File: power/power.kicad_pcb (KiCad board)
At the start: 2 copper layers, 49.5 x 48.3 mm, 7 parts, among them J1 Conn_01x08_Male, J2 Conn_01x08_Male, J3 Jack-DC

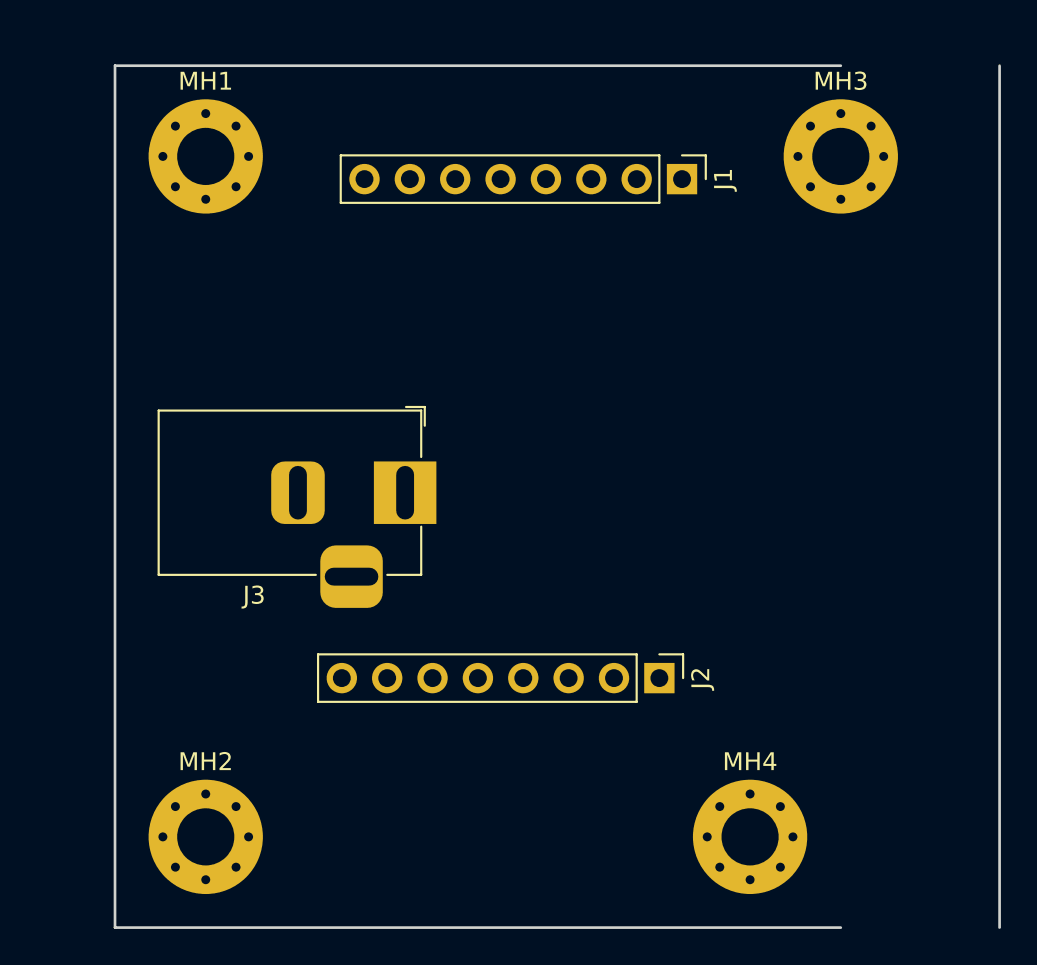
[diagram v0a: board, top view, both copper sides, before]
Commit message: Ready
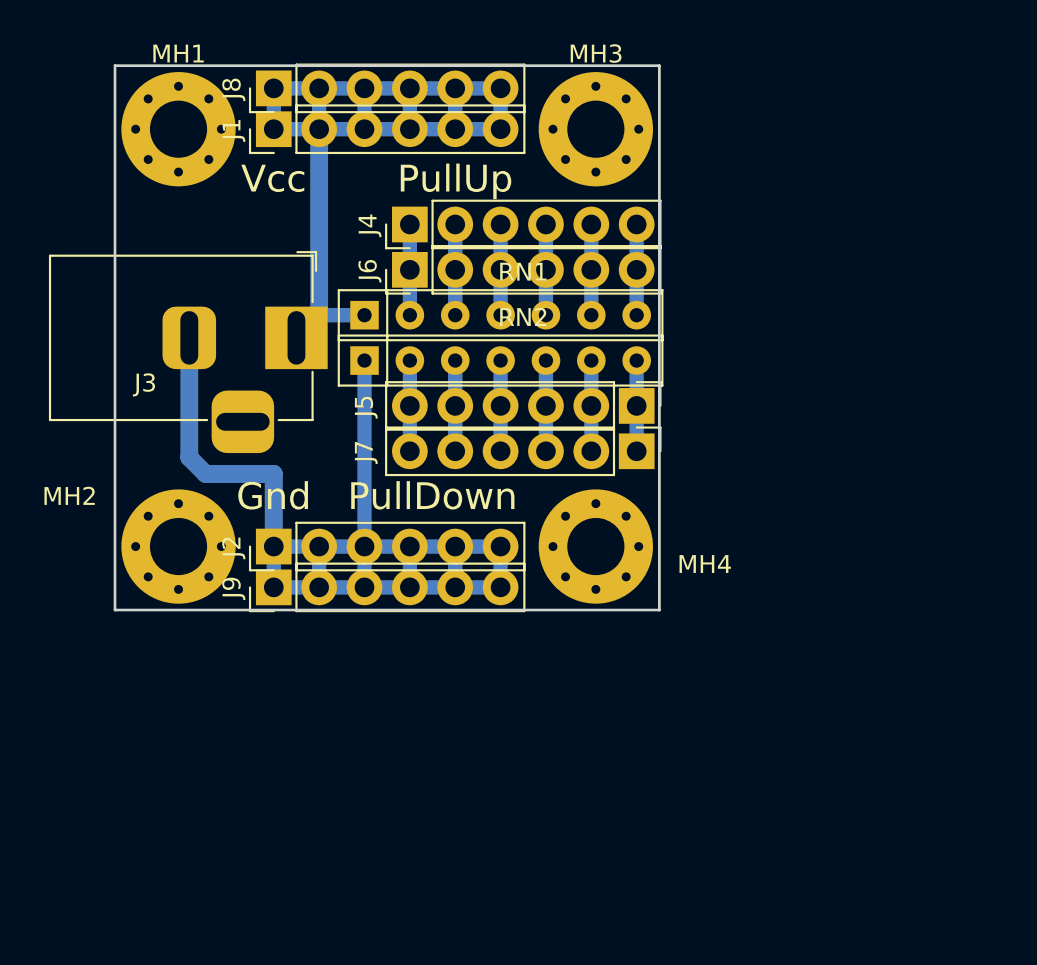
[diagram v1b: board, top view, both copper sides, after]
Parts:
- added J4: Conn_01x06_Male, MyLib:PinHeader_1x06_P2.54mm_Vertical_BigHoles, F.Cu at (148.6, 43.2)
- added J5: Conn_01x06_Male, MyLib:PinHeader_1x06_P2.54mm_Vertical_BigHoles, F.Cu at (161.3, 53.3)
- added J6: Conn_01x06_Male, MyLib:PinHeader_1x06_P2.54mm_Vertical_BigHoles, F.Cu at (148.6, 45.7)
- added J7: Conn_01x06_Male, MyLib:PinHeader_1x06_P2.54mm_Vertical_BigHoles, F.Cu at (161.3, 55.9)
- added J8: Conn_01x06_Male, MyLib:PinHeader_1x06_P2.54mm_Vertical_BigHoles, F.Cu at (141.0, 35.6)
- added J9: Conn_01x06_Male, MyLib:PinHeader_1x06_P2.54mm_Vertical_BigHoles, F.Cu at (141.0, 63.5)
- added RN1: R_Network06, Resistor_THT:R_Array_SIP7, F.Cu at (146.1, 48.3)
- added RN2: R_Network06, Resistor_THT:R_Array_SIP7, F.Cu at (146.1, 50.8)
- J1, J2: value Conn_01x08_Male -> Conn_01x06_Male; footprint Connector_PinHeader_2.54mm:PinHeader_1x08_P2.54mm_Vertical -> MyLib:PinHeader_1x06_P2.54mm_Vertical_BigHoles
- moved J1 23.0 mm to (141.0, 37.8), turned to 90 degrees
- moved J2 22.8 mm to (141.0, 61.2), turned to 90 degrees
- moved MH4 18.4 mm to (159.0, 61.2)
- moved MH2 16.3 mm to (135.6, 61.2)
- moved MH3 13.8 mm to (159.0, 37.8)
- moved J3 10.6 mm to (142.2, 49.5)
- moved MH1 2.16 mm to (135.6, 37.8)
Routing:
- net GND: track 0.00 -> 65.4 mm
- net VCC: track 0.00 -> 53.9 mm
- net Net-(J5-Pad6): track 0.00 -> 5.08 mm
- net Net-(J5-Pad5): track 0.00 -> 5.08 mm
- net Net-(J5-Pad4): track 0.00 -> 5.08 mm
- net Net-(J5-Pad3): track 0.00 -> 5.08 mm
- net Net-(J5-Pad2): track 0.00 -> 5.08 mm
- net Net-(J5-Pad1): track 0.00 -> 5.08 mm
- net Net-(J4-Pad6): track 0.00 -> 5.08 mm
- net Net-(J4-Pad5): track 0.00 -> 5.08 mm
- net Net-(J4-Pad4): track 0.00 -> 5.08 mm
- net Net-(J4-Pad3): track 0.00 -> 5.08 mm
- net Net-(J4-Pad2): track 0.00 -> 5.08 mm
- net Net-(J4-Pad1): track 0.00 -> 5.08 mm
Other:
- board size 49.5 x 48.3 mm -> 30.5 x 30.5 mm
- board text added: "Gnd"
- board text added: "PullDown"
- board text added: "PullUp"
- board text added: "Vcc"
